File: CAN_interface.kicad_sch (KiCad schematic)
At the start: 24 parts, among them J3 CAN_OUT, J4 CAN_IN, U4 MCP2515-xST, U5 MCP2551-I-SN, Y3 Crystal_GND24

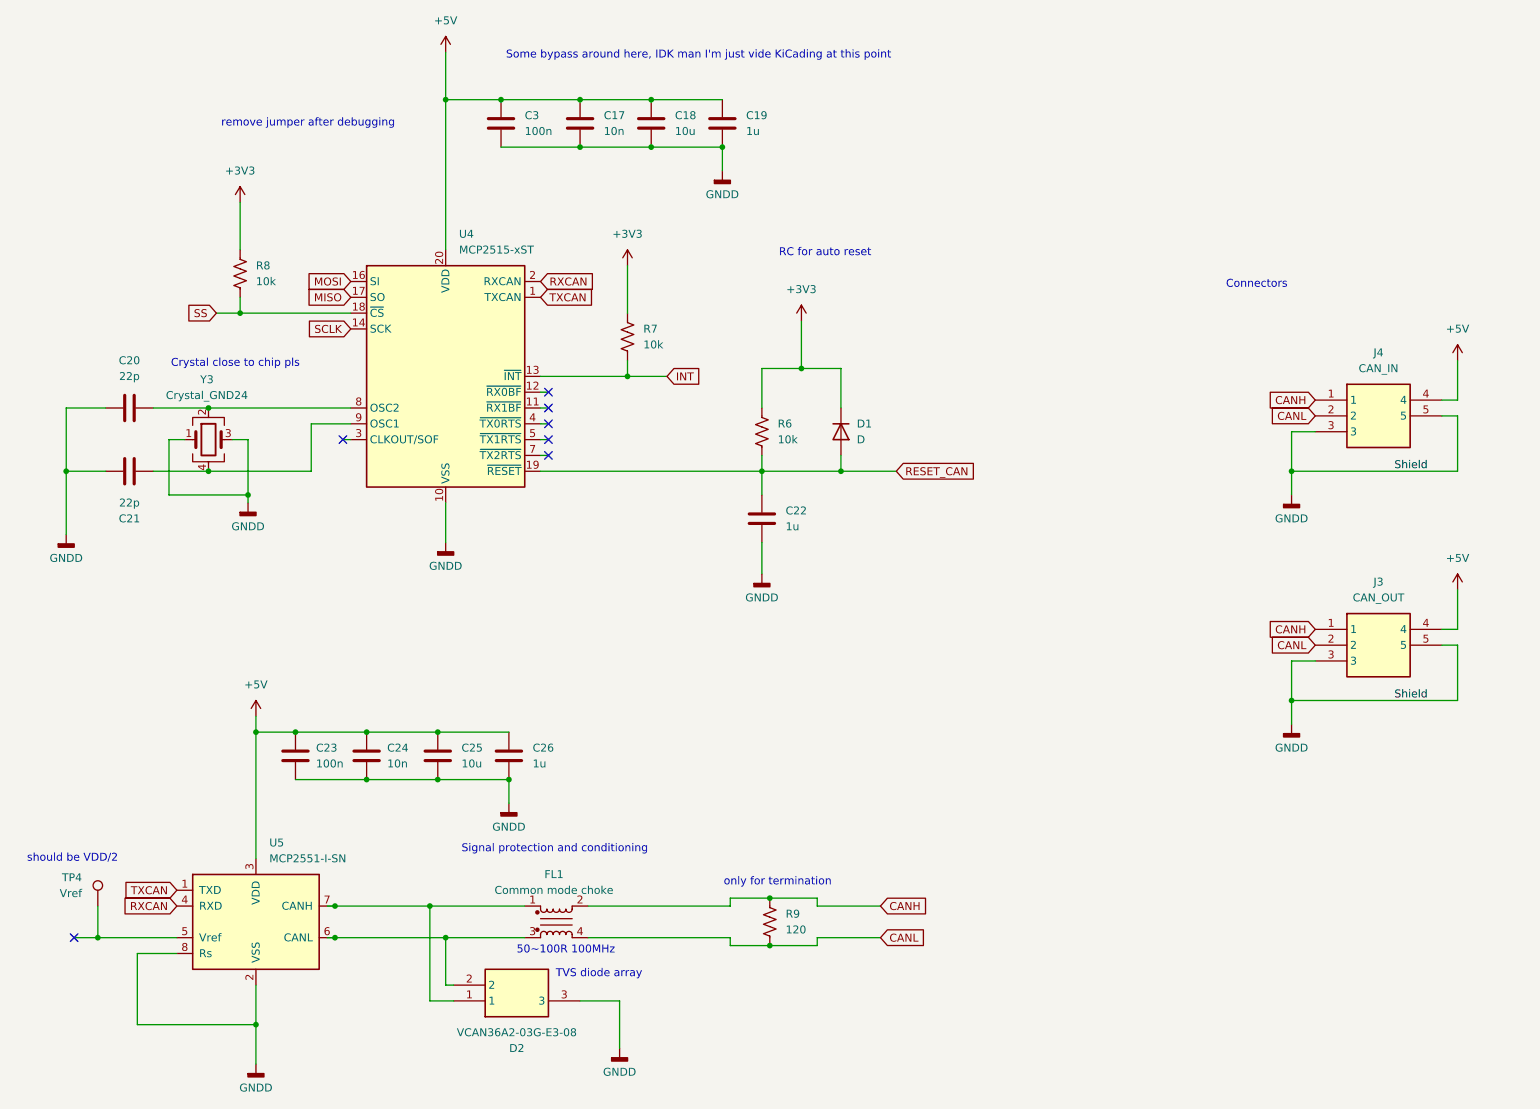
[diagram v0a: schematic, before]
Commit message: changed the mcp - potentiellement final version
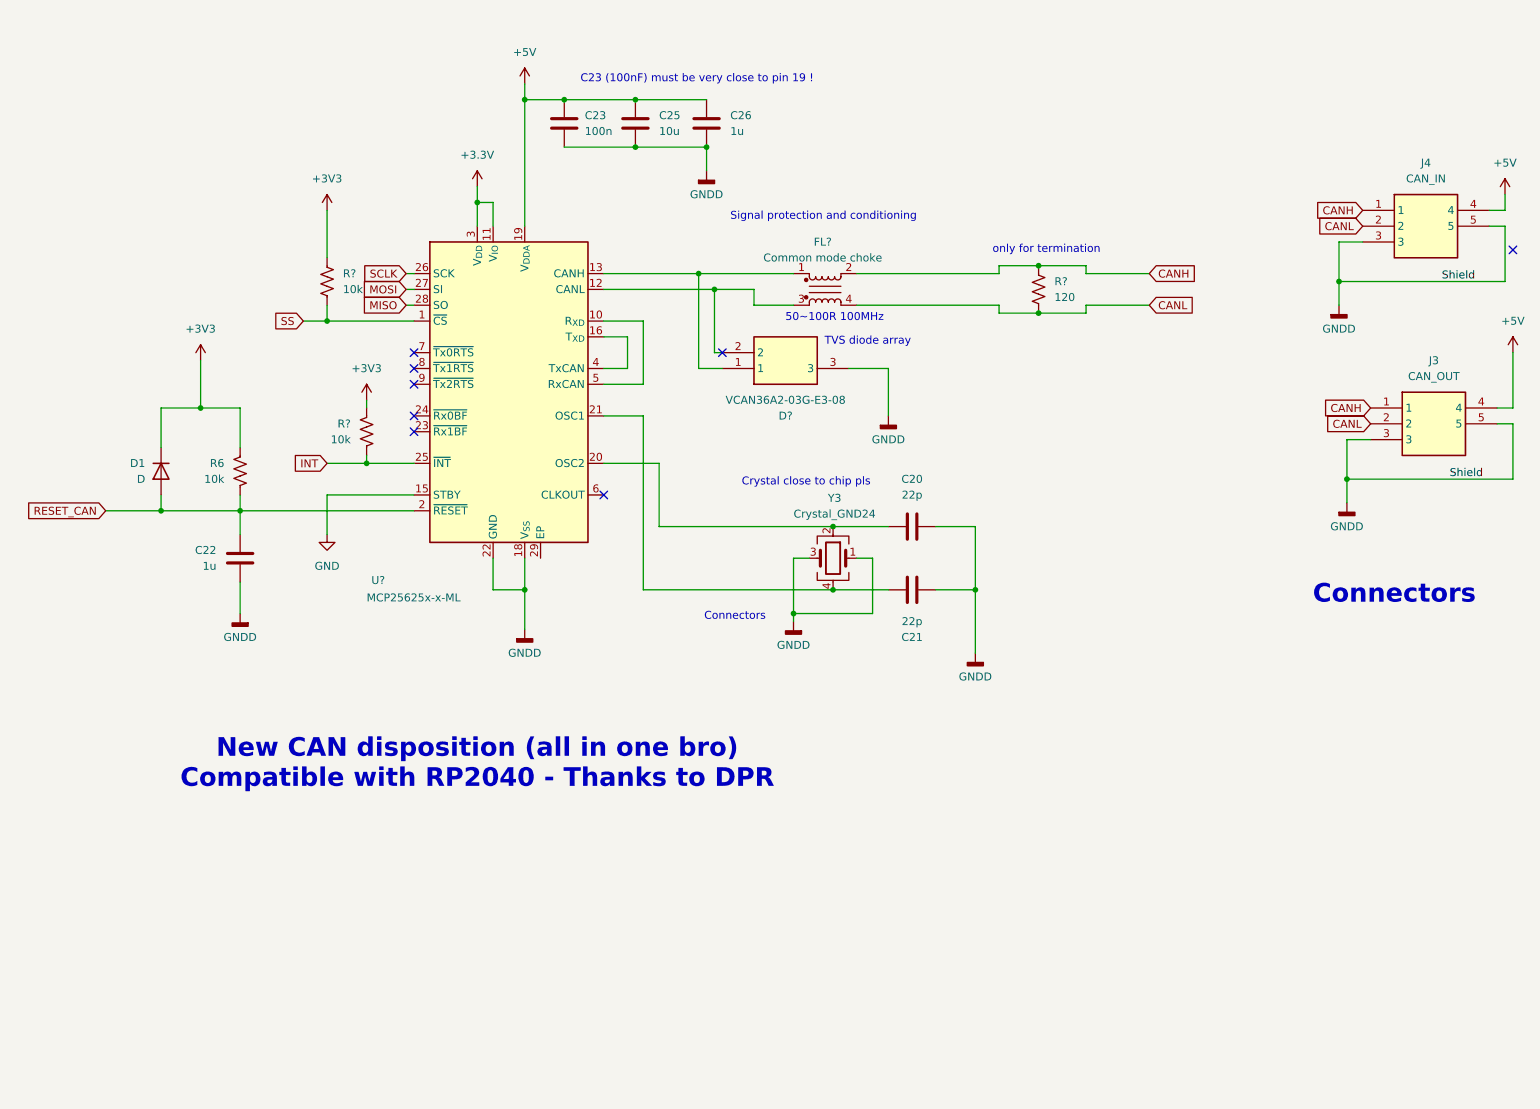
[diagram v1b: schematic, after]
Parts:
- removed C17, C24: 10n, Capacitor_SMD:C_0402_1005Metric, symbol Device:C
- removed C18: 10u, Capacitor_SMD:C_0805_2012Metric, symbol Device:C
- removed C19: 1u, Capacitor_SMD:C_0603_1608Metric, symbol Device:C
- removed C3: 100n, Capacitor_SMD:C_0402_1005Metric, symbol Device:C
- removed D2: VCAN36A2-03G-E3-08, KiNic_footprints:SOT65P230X110-3N, symbol KiNic_symbols:VCAN36A2-03G-E3-08
- removed FL1: Common mode choke, KiNic_footprints:DLW21SN121HQ2L, symbol Device:Filter_EMI_CommonMode
- removed R7, R8: 10k, Resistor_SMD:R_0603_1608Metric, symbol Device:R_US
- removed R9: 120, Resistor_SMD:R_0603_1608Metric, symbol Device:R_US
- removed TP4: Vref, TestPoint:TestPoint_Pad_D2.0mm, symbol Connector:TestPoint
- removed U4: MCP2515-xST, Package_SO:TSSOP-20_4.4x6.5mm_P0.65mm, symbol Interface_CAN_LIN:MCP2515-xST
- removed U5: MCP2551-I-SN, Package_SO:SOIC-8_3.9x4.9mm_P1.27mm, symbol Interface_CAN_LIN:MCP2551-I-SN
- added D?: VCAN36A2-03G-E3-08, KiNic_footprints:SOT65P230X110-3N, symbol KiNic_symbols:VCAN36A2-03G-E3-08
- added FL?: Common mode choke, KiNic_footprints:DLW21SN121HQ2L, symbol Device:Filter_EMI_CommonMode
- added R?: 120, Resistor_SMD:R_0603_1608Metric, symbol Device:R_US
- added R? (x2): 10k, Resistor_SMD:R_0603_1608Metric, symbol Device:R_US
- added U?: MCP25625x-x-ML, Package_DFN_QFN:QFN-28-1EP_6x6mm_P0.65mm_EP4.25x4.25mm, symbol Interface_CAN_LIN:MCP25625x-x-ML
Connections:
- net +3V3: now also R?.1, R?.1
- net +5V: now also U?.19 (V_{DDA})
- net CANH: now also FL?.2, R?.1
- net CANL: now also FL?.4, R?.2
- net GNDD: now also D?.3, U?.18 (V_{SS}), U?.22 (GND)
- net INT: now also R?.2, U?.25 (~{INT})
- net MISO: now also U?.28 (SO)
- net MOSI: now also U?.27 (SI)
- net RESET_CAN: now also U?.2 (~{RESET})
- net SCLK: now also U?.26 (SCK)
- net SS: now also R?.2, U?.1 (~{CS})
- net at C20.1, Y3.2: now also U?.20 (OSC2)
- net at C21.1, Y3.4: now also U?.21 (OSC1)
- new net: D?.1, FL?.1, U?.13 (CANH)
- new net: D?.2, FL?.3, U?.12 (CANL)
- new net: U?.10 (R_{XD}), U?.5 (RxCAN)
- new net: U?.16 (T_{XD}), U?.4 (TxCAN)
- new net +3.3V: U?.11 (V_{IO}), U?.3 (V_{DD})
- new net GND: U?.15 (STBY)
- no-connect marks 7 -> 8
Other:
- note added: "C23 (100nF) must be very close to pin 19 !"
- note added: "New CAN disposition (all in one bro) Compatible with RP2040 - Thanks to DPR"
- note removed: "RC for auto reset"
- note removed: "Some bypass around here, IDK man I'm just vide KiCading at this point"
- note removed: "remove jumper after debugging"
- note removed: "should be VDD/2"
- moved on the sheet: C20, C21, C22, C23, C25, C26, D1, J3, J4, R6, Y3
